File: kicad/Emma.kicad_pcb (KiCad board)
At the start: 4 copper layers, 55 x 35 mm, 75 parts, among them U1 ByA 100nF +3V3 U1-VDDA Bypass, U1 ByB 100nF +3V3 U1-VDD Bypass

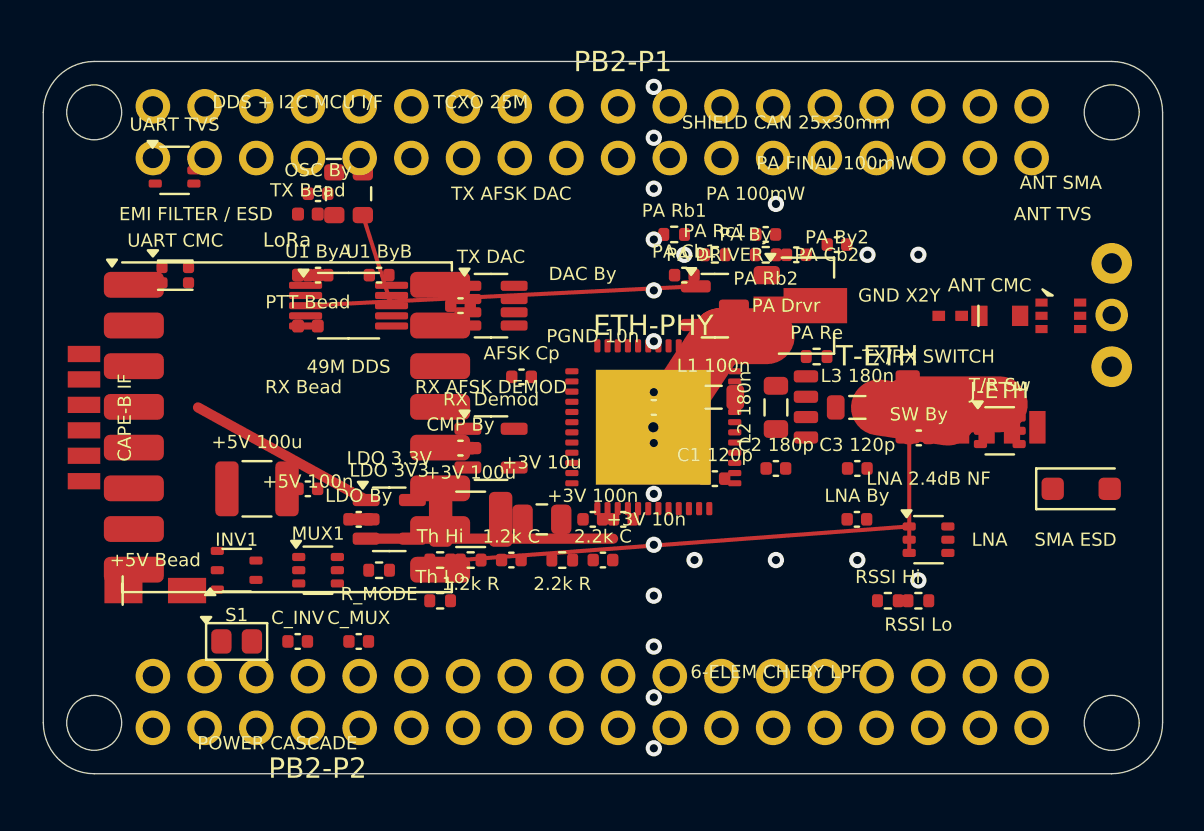
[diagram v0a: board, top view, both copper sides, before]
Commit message: updated avionics and docs
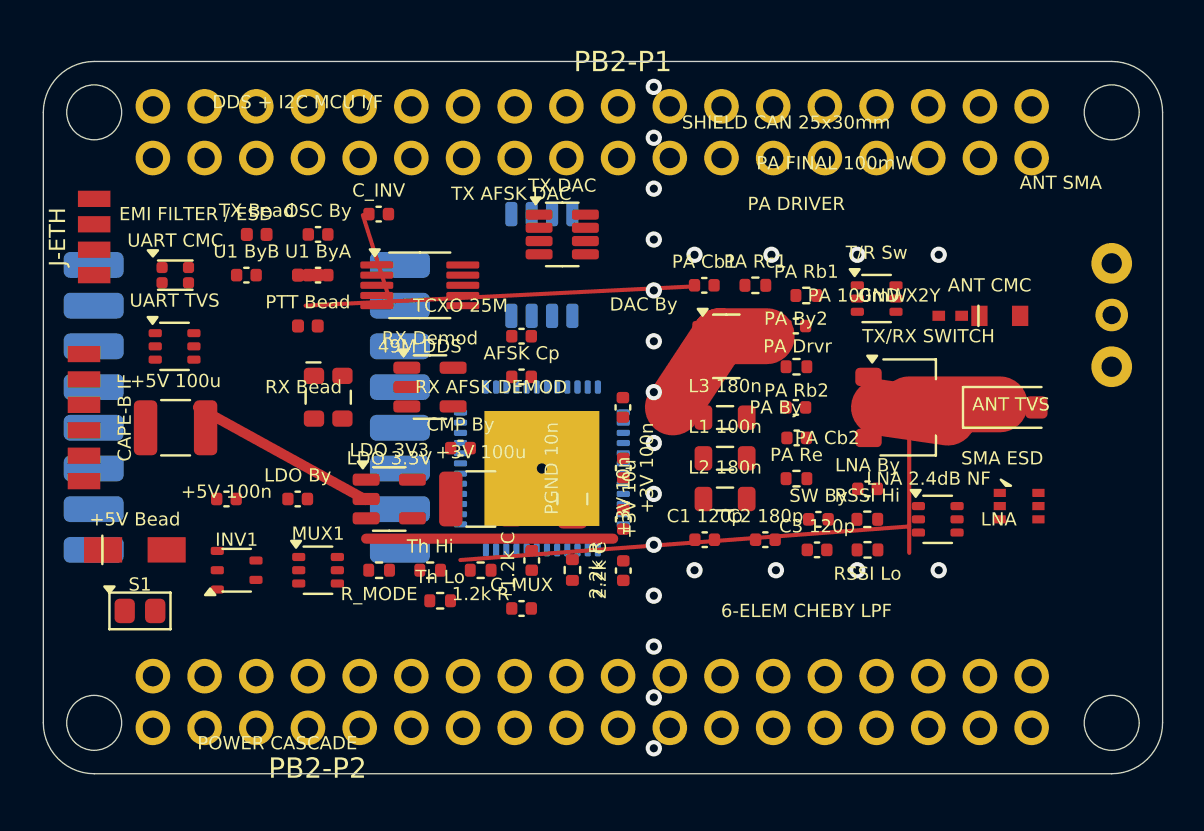
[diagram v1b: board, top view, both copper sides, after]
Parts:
- ETH-PHY, LoRa, T-ETH: moved to B.Cu
- moved J-ETH 45.4 mm to (102.5, 108.6), turned to 90 degrees
- moved C_INV 21.4 mm to (116.5, 107.5)
- moved T-ETH 17.0 mm to (124.5, 110.0), turned to 90 degrees
- moved TCXO 25M 10.0 mm to (114.0, 116.5)
- moved ANT TVS 9.57 mm to (147.9, 121.8)
- moved PA Cb2 9.00 mm to (137.0, 118.5)
- moved T/R Sw 8.88 mm to (140.9, 111.7)
- moved UART TVS 8.65 mm to (106.5, 114.0)
- moved PA By 8.63 mm to (137.0, 117.0)
- moved C_MUX 8.16 mm to (123.5, 126.9)
- moved PA Rb1 7.15 mm to (137.5, 111.5)
- moved PA 100mW 7.07 mm to (142.5, 117.0)
- moved U1 ByB 6.52 mm to (110.0, 110.5)
- moved L3 180n 6.52 mm to (133.5, 117.5)
- moved SW By 6.35 mm to (138.1, 122.5)
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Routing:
- net GND: track 0.00 -> 57.6 mm
- net RX_LNA: track 22.1 -> 0.00 mm
- net +3V3: track 12.1 -> 0.00 mm
- net +5V_FILT: track 9.43 -> 0.00 mm
- net RF_RX: track 6.00 -> 0.00 mm
- net RF_ANT_SW: track 4.45 -> 0.00 mm
- net RF_FILT: track 3.42 -> 0.00 mm
